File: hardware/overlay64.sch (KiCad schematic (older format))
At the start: 17 parts, among them IC1 ATMEGA328P-P, P1 ISP, P2 MAIN, P3 INPUT/BYPASS, Q1 BC547B, U1 LM1881, Y1 20MHz

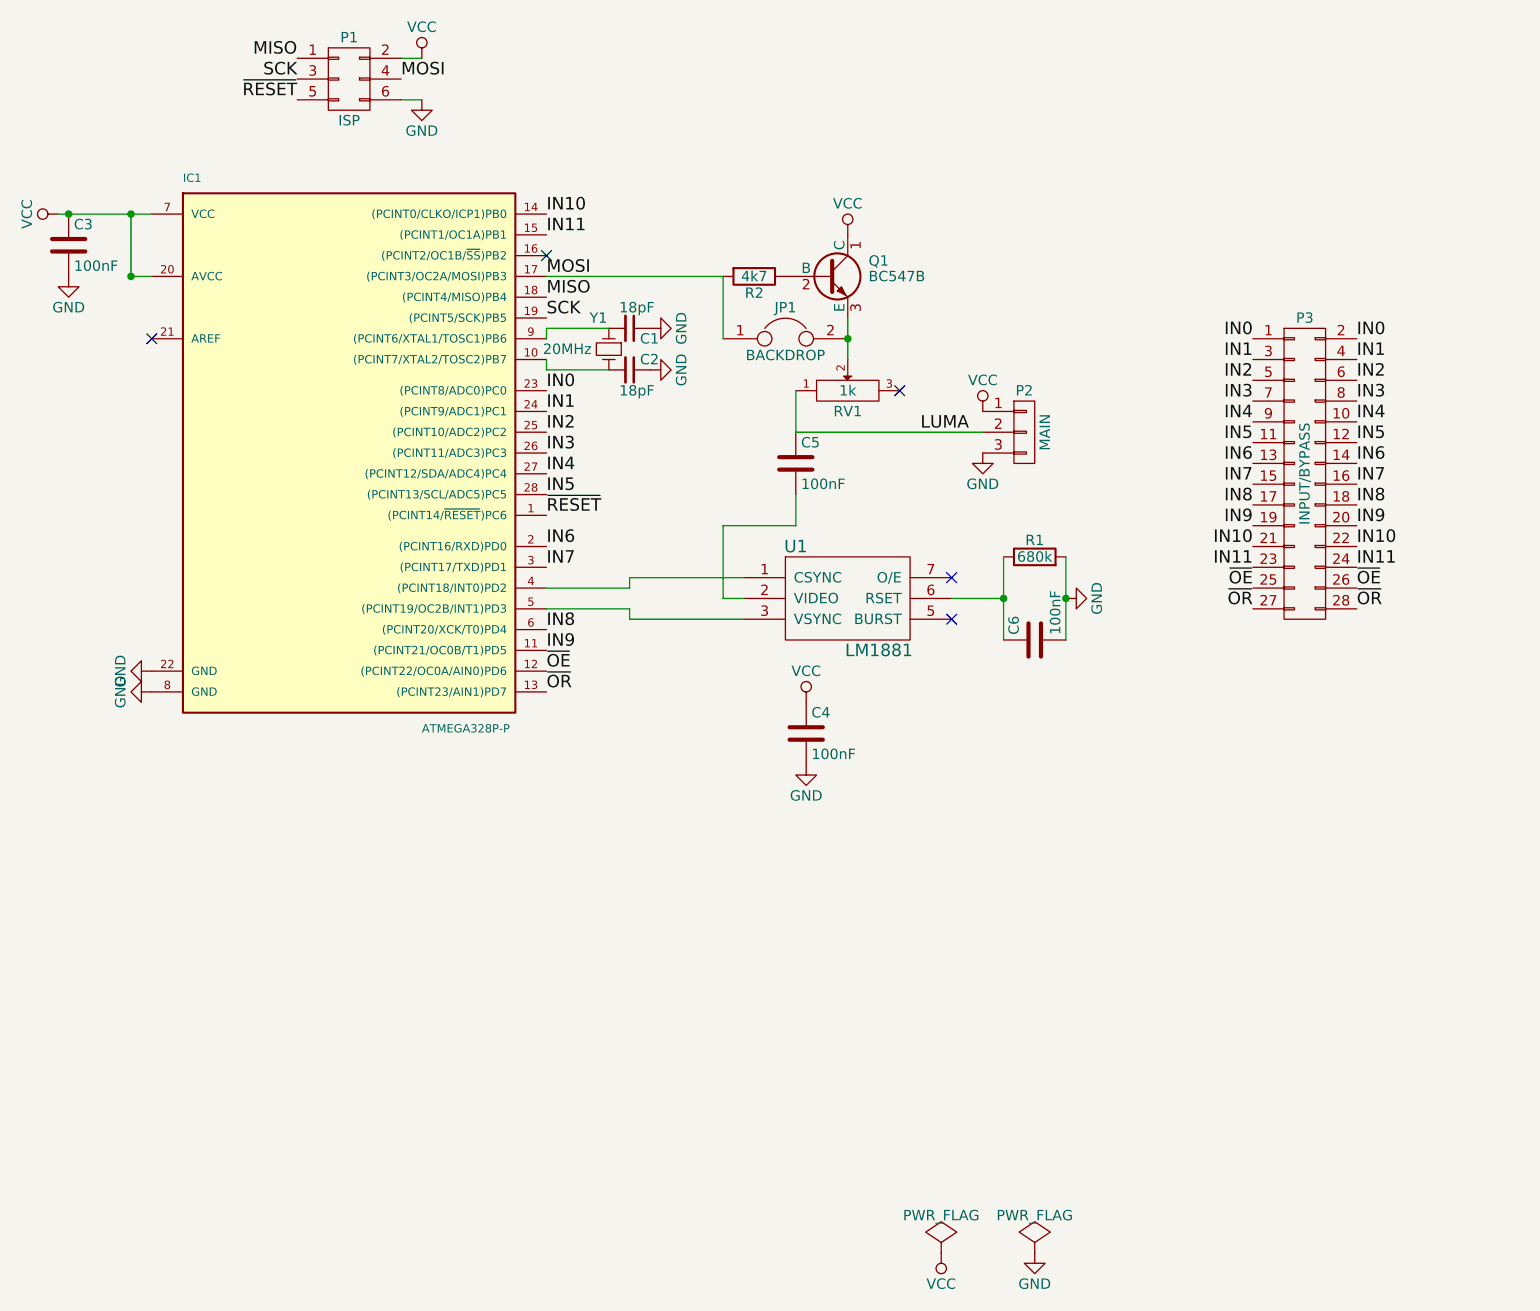
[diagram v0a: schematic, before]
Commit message: Hardware: Rearranged components, rerouting...
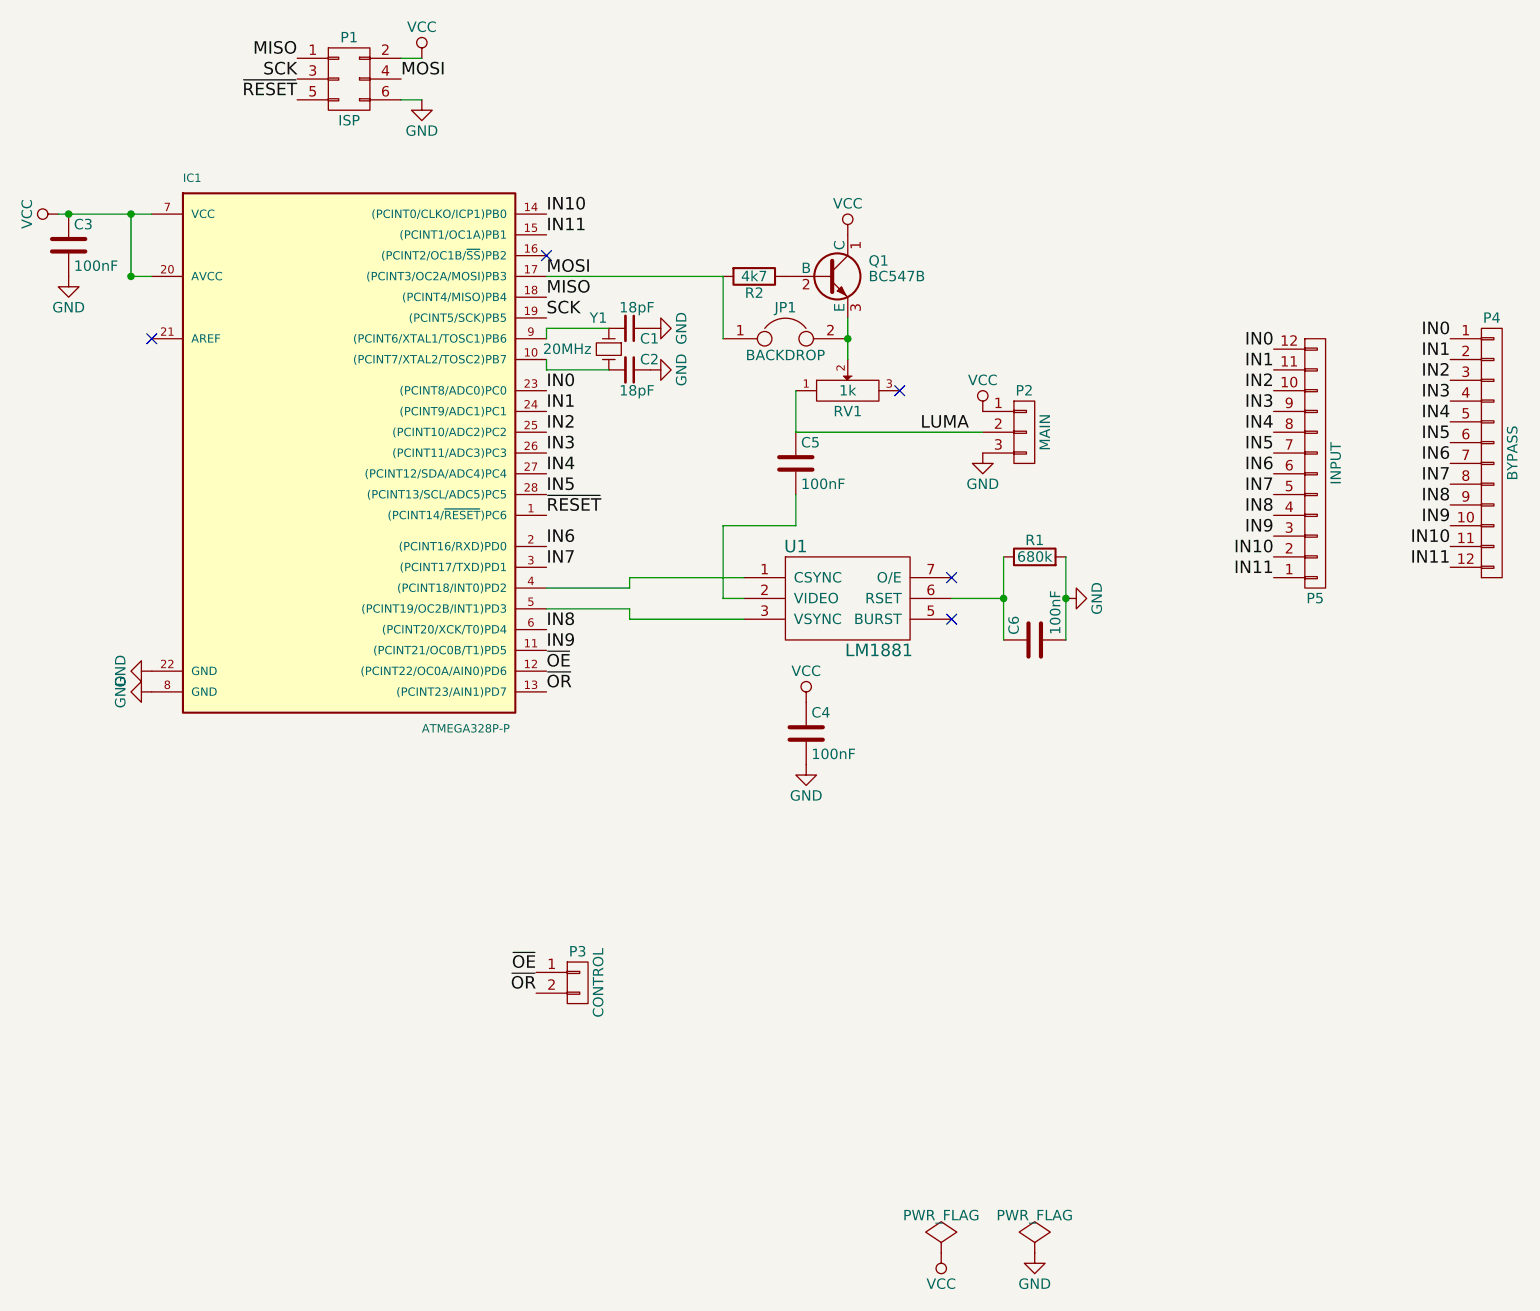
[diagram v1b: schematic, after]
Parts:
- removed P3: INPUT/BYPASS, Pin_Headers:Pin_Header_Straight_2x14, symbol CONN_02X14
- added P3: CONTROL, Pin_Headers:Pin_Header_Angled_1x02, symbol CONN_01X02
- added P4: BYPASS, Pin_Headers:Pin_Header_Angled_1x12, symbol CONN_01X12
- added P5: INPUT, Pin_Headers:Pin_Header_Angled_1x12, symbol CONN_01X12
- P2: footprint Pin_Headers:Pin_Header_Straight_1x03 -> Pin_Headers:Pin_Header_Angled_1x03
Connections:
- net IN0: now also P4.1 (P1), P5.12 (P12)
- net IN1: now also P4.2 (P2), P5.11 (P11)
- net IN10: now also P4.11 (P11), P5.2 (P2)
- net IN11: now also P4.12 (P12), P5.1 (P1)
- net IN2: now also P4.3 (P3), P5.10 (P10)
- net IN3: now also P4.4 (P4), P5.9 (P9)
- net IN4: now also P4.5 (P5), P5.8 (P8)
- net IN5: now also P4.6 (P6), P5.7 (P7)
- net IN6: now also P4.7 (P7), P5.6 (P6)
- net IN7: now also P4.8 (P8), P5.5 (P5)
- net IN8: now also P4.9 (P9), P5.4 (P4)
- net IN9: now also P4.10 (P10), P5.3 (P3)
- net ~OE: now also P3.1 (P1)
- net ~OR: now also P3.2 (P2)
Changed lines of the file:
@@
 $EndComp
 $Comp
-L PWR_FLAG #FLG1
+L PWR_FLAG #FLG01
 U 1 1 56A1EF0B
 P 6250 7500
-F 0 "#FLG1" H 6250 7595 50  0001 C CNN
+F 0 "#FLG01" H 6250 7595 50  0001 C CNN
 F 1 "PWR_FLAG" H 6250 7680 50  0000 C CNN
 F 2 "" H 6250 7500 60  0000 C CNN
@@
 $EndComp
 $Comp
-L VCC #PWR12
+L VCC #PWR02
 U 1 1 56A1EF40
 P 6250 7500
-F 0 "#PWR12" H 6250 7350 50  0001 C CNN
+F 0 "#PWR02" H 6250 7350 50  0001 C CNN
 F 1 "VCC" H 6250 7650 50  0000 C CNN
 F 2 "" H 6250 7500 60  0000 C CNN
@@
 $EndComp
 $Comp
-L PWR_FLAG #FLG2
+L PWR_FLAG #FLG03
 U 1 1 56A1EF56
 P 6700 7500
-F 0 "#FLG2" H 6700 7595 50  0001 C CNN
+F 0 "#FLG03" H 6700 7595 50  0001 C CNN
 F 1 "PWR_FLAG" H 6700 7680 50  0000 C CNN
 F 2 "" H 6700 7500 60  0000 C CNN
@@
 $EndComp
 $Comp
-L GND #PWR15
+L GND #PWR04
 U 1 1 56A1EF6C
 P 6700 7500
-F 0 "#PWR15" H 6700 7250 50  0001 C CNN
+F 0 "#PWR04" H 6700 7250 50  0001 C CNN
 F 1 "GND" H 6700 7350 50  0000 C CNN
 F 2 "" H 6700 7500 60  0000 C CNN
@@
 $EndComp
 $Comp
-L VCC #PWR9
+L VCC #PWR05
 U 1 1 56A1F13D
 P 5600 4850
-F 0 "#PWR9" H 5600 4700 50  0001 C CNN
+F 0 "#PWR05" H 5600 4700 50  0001 C CNN
 F 1 "VCC" H 5600 5000 50  0000 C CNN
 F 2 "" H 5600 4850 60  0000 C CNN
@@
 $EndComp
 $Comp
-L GND #PWR10
+L GND #PWR06
 U 1 1 56A1F155
 P 5600 5150
-F 0 "#PWR10" H 5600 4900 50  0001 C CNN
+F 0 "#PWR06" H 5600 4900 50  0001 C CNN
 F 1 "GND" H 5600 5000 50  0000 C CNN
 F 2 "" H 5600 5150 60  0000 C CNN
@@
 $EndComp
 $Comp
-L GND #PWR2
+L GND #PWR07
 U 1 1 56A1F1BC
 P 2050 2800
-F 0 "#PWR2" H 2050 2550 50  0001 C CNN
+F 0 "#PWR07" H 2050 2550 50  0001 C CNN
 F 1 "GND" H 2050 2650 50  0000 C CNN
 F 2 "" H 2050 2800 60  0000 C CNN
@@
 $EndComp
 $Comp
-L GND #PWR16
+L GND #PWR08
 U 1 1 56A1F3BB
 P 6850 4350
-F 0 "#PWR16" H 6850 4100 50  0001 C CNN
+F 0 "#PWR08" H 6850 4100 50  0001 C CNN
 F 1 "GND" H 6850 4200 50  0000 C CNN
 F 2 "" H 6850 4350 60  0000 C CNN
@@
 $EndComp
 $Comp
-L VCC #PWR1
+L VCC #PWR09
 U 1 1 56A1FF3A
 P 2000 2500
-F 0 "#PWR1" H 2000 2350 50  0001 C CNN
+F 0 "#PWR09" H 2000 2350 50  0001 C CNN
 F 1 "VCC" H 2000 2650 50  0000 C CNN
 F 2 "" H 2000 2500 60  0000 C CNN
@@
 $EndComp
 $Comp
-L GND #PWR3
+L GND #PWR010
 U 1 1 56A20155
 P 2450 4700
-F 0 "#PWR3" H 2450 4450 50  0001 C CNN
+F 0 "#PWR010" H 2450 4450 50  0001 C CNN
 F 1 "GND" H 2450 4550 50  0000 C CNN
 F 2 "" H 2450 4700 60  0000 C CNN
@@
 $EndComp
 $Comp
-L GND #PWR4
+L GND #PWR011
 U 1 1 56A60DBD
 P 2450 4800
-F 0 "#PWR4" H 2450 4550 50  0001 C CNN
+F 0 "#PWR011" H 2450 4550 50  0001 C CNN
 F 1 "GND" H 2450 4650 50  0000 C CNN
 F 2 "" H 2450 4800 60  0000 C CNN
@@
 Connection ~ 6850 4350
 $Comp
-L VCC #PWR11
+L VCC #PWR012
 U 1 1 56A78618
 P 5800 2600
-F 0 "#PWR11" H 5800 2450 50  0001 C CNN
+F 0 "#PWR012" H 5800 2450 50  0001 C CNN
 F 1 "VCC" H 5800 2750 50  0000 C CNN
 F 2 "" H 5800 2600 60  0000 C CNN
@@
 MOSI
 $Comp
-L VCC #PWR5
+L VCC #PWR013
 U 1 1 56A92B5A
 P 3750 1750
-F 0 "#PWR5" H 3750 1600 50  0001 C CNN
+F 0 "#PWR013" H 3750 1600 50  0001 C CNN
 F 1 "VCC" H 3750 1900 50  0000 C CNN
 F 2 "" H 3750 1750 60  0000 C CNN
@@
 $EndComp
 $Comp
-L GND #PWR6
+L GND #PWR014
 U 1 1 56A92BBD
 P 3750 1950
-F 0 "#PWR6" H 3750 1700 50  0001 C CNN
+F 0 "#PWR014" H 3750 1700 50  0001 C CNN
 F 1 "GND" H 3750 1800 50  0000 C CNN
 F 2 "" H 3750 1950 60  0000 C CNN
@@
 $EndComp
 $Comp
-L GND #PWR7
+L GND #PWR015
 U 1 1 56A976F1
 P 4850 3050
-F 0 "#PWR7" H 4850 2800 50  0001 C CNN
+F 0 "#PWR015" H 4850 2800 50  0001 C CNN
 F 1 "GND" H 4850 2900 50  0000 C CNN
 F 2 "" H 4850 3050 60  0000 C CNN
@@
 $EndComp
 $Comp
-L GND #PWR8
+L GND #PWR016
 U 1 1 56A97733
 P 4850 3250
-F 0 "#PWR8" H 4850 3000 50  0001 C CNN
+F 0 "#PWR016" H 4850 3000 50  0001 C CNN
 F 1 "GND" H 4850 3100 50  0000 C CNN
 F 2 "" H 4850 3250 60  0000 C CNN
@@
 F 0 "P2" H 6650 3750 50  0000 C CNN
 F 1 "MAIN" V 6750 3550 50  0000 C CNN
-F 2 "Pin_Headers:Pin_Header_Straight_1x03" H 6650 3550 60  0001 C CNN
+F 2 "Pin_Headers:Pin_Header_Angled_1x03" H 6650 3550 60  0001 C CNN
 F 3 "" H 6650 3550 60  0000 C CNN
 	1    6650 3550
@@
 $EndComp
 $Comp
-L VCC #PWR13
+L VCC #PWR017
 U 1 1 56A9E7D0
 P 6450 3450
-F 0 "#PWR13" H 6450 3300 50  0001 C CNN
+F 0 "#PWR017" H 6450 3300 50  0001 C CNN
 F 1 "VCC" H 6450 3600 50  0000 C CNN
 F 2 "" H 6450 3450 60  0000 C CNN
@@
 $EndComp
 $Comp
-L GND #PWR14
+L GND #PWR018
 U 1 1 56A9E875
 P 6450 3650
-F 0 "#PWR14" H 6450 3400 50  0001 C CNN
+F 0 "#PWR018" H 6450 3400 50  0001 C CNN
 F 1 "GND" H 6450 3500 50  0000 C CNN
 F 2 "" H 6450 3650 60  0000 C CNN
@@
 Wire Wire Line
 	4750 4450 5300 4450
-Text Label 7750 3100 2    60   ~ 0
+Text Label 8700 3100 2    60   ~ 0
 IN0
-Text Label 7750 3200 2    60   ~ 0
+Text Label 8700 3200 2    60   ~ 0
 IN1
-Text Label 7750 3300 2    60   ~ 0
+Text Label 8700 3300 2    60   ~ 0
 IN2
-Text Label 7750 3400 2    60   ~ 0
+Text Label 8700 3400 2    60   ~ 0
 IN3
-Text Label 7750 3500 2    60   ~ 0
+Text Label 8700 3500 2    60   ~ 0
 IN4
-Text Label 7750 3600 2    60   ~ 0
+Text Label 8700 3600 2    60   ~ 0
 IN5
-Text Label 7750 3700 2    60   ~ 0
+Text Label 8700 3700 2    60   ~ 0
 IN6
-Text Label 7750 3800 2    60   ~ 0
+Text Label 8700 3800 2    60   ~ 0
 IN7
-Text Label 7750 3900 2    60   ~ 0
+Text Label 8700 3900 2    60   ~ 0
 IN8
-Text Label 7750 4000 2    60   ~ 0
+Text Label 8700 4000 2    60   ~ 0
 IN9
-Text Label 7750 4100 2    60   ~ 0
+Text Label 8700 4100 2    60   ~ 0
 IN10
-Text Label 7750 4200 2    60   ~ 0
+Text Label 8700 4200 2    60   ~ 0
 IN11
 $Comp
@@
 Text Label 4350 4800 0    60   ~ 0
 ~OR
-Text Label 7750 4300 2    60   ~ 0
+Text Label 4300 6150 2    60   ~ 0
 ~OE
 Text Label 6150 3550 0    60   ~ 0
 LUMA
-$Comp
-L CONN_02X14 P3
-U 1 1 56B0DCD2
-P 8000 3750
-F 0 "P3" H 8000 4500 50  0000 C CNN
-F 1 "INPUT/BYPASS" V 8000 3750 50  0000 C CNN
-F 2 "Pin_Headers:Pin_Header_Straight_2x14" H 8000 2600 60  0001 C CNN
-F 3 "" H 8000 2600 60  0000 C CNN
-	1    8000 3750
-	1    0    0    -1
-$EndComp
-Text Label 8250 4300 0    60   ~ 0
-~OE
-Text Label 8250 3100 0    60   ~ 0
+Text Label 7850 3150 2    60   ~ 0
 IN0
-Text Label 8250 3200 0    60   ~ 0
+Text Label 7850 3250 2    60   ~ 0
 IN1
-Text Label 8250 3300 0    60   ~ 0
+Text Label 7850 3350 2    60   ~ 0
 IN2
-Text Label 8250 3400 0    60   ~ 0
+Text Label 7850 3450 2    60   ~ 0
 IN3
-Text Label 8250 3500 0    60   ~ 0
+Text Label 7850 3550 2    60   ~ 0
 IN4
-Text Label 8250 3600 0    60   ~ 0
+Text Label 7850 3650 2    60   ~ 0
 IN5
-Text Label 8250 3700 0    60   ~ 0
+Text Label 7850 3750 2    60   ~ 0
 IN6
-Text Label 8250 3800 0    60   ~ 0
+Text Label 7850 3850 2    60   ~ 0
 IN7
-Text Label 8250 3900 0    60   ~ 0
+Text Label 7850 3950 2    60   ~ 0
 IN8
-Text Label 8250 4000 0    60   ~ 0
+Text Label 7850 4050 2    60   ~ 0
 IN9
-Text Label 8250 4100 0    60   ~ 0
+Text Label 7850 4150 2    60   ~ 0
 IN10
-Text Label 8250 4200 0    60   ~ 0
+Text Label 7850 4250 2    60   ~ 0
 IN11
 $Comp
@@
 Text Label 4350 4700 0    60   ~ 0
 ~OE
-Text Label 8250 4400 0    60   ~ 0
+Text Label 4300 6250 2    60   ~ 0
 ~OR
-Text Label 7750 4400 2    60   ~ 0
-~OR
+$Comp
+L CONN_01X12 P4
+U 1 1 572F57F1
+P 8900 3650
+F 0 "P4" H 8900 4300 50  0000 C CNN
+F 1 "BYPASS" V 9000 3650 50  0000 C CNN
+F 2 "Pin_Headers:Pin_Header_Angled_1x12" H 8900 3650 50  0001 C CNN
+F 3 "" H 8900 3650 50  0000 C CNN
+	1    8900 3650
+	1    0    0    -1
+$EndComp
+$Comp
+L CONN_01X12 P5
+U 1 1 572F58A5
+P 8050 3700
+F 0 "P5" H 8050 4350 50  0000 C CNN
+F 1 "INPUT" V 8150 3700 50  0000 C CNN
+F 2 "Pin_Headers:Pin_Header_Angled_1x12" H 8050 3700 50  0001 C CNN
+F 3 "" H 8050 3700 50  0000 C CNN
+	1    8050 3700
+	1    0    0    1
+$EndComp
+$Comp
+L CONN_01X02 P3
+U 1 1 572F59E5
+P 4500 6200
+F 0 "P3" H 4500 6350 50  0000 C CNN
+F 1 "CONTROL" V 4600 6200 50  0000 C CNN
+F 2 "Pin_Headers:Pin_Header_Angled_1x02" H 4500 6200 50  0001 C CNN
+F 3 "" H 4500 6200 50  0000 C CNN
+	1    4500 6200
+	1    0    0    -1
+$EndComp
 $EndSCHEMATC
